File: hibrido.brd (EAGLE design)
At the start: 84 x 80 mm, 30 parts

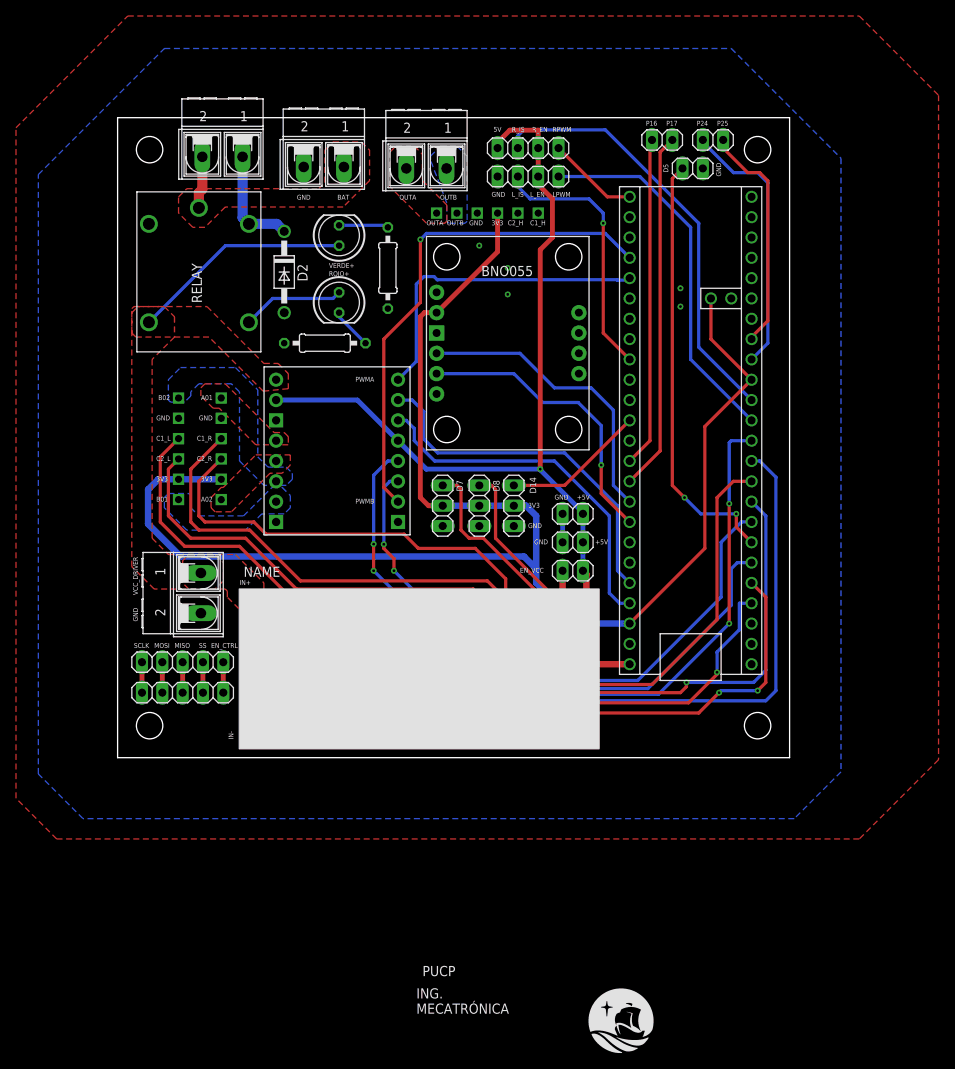
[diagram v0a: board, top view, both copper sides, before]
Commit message: Version final de la PCB, falta revisar por los demás
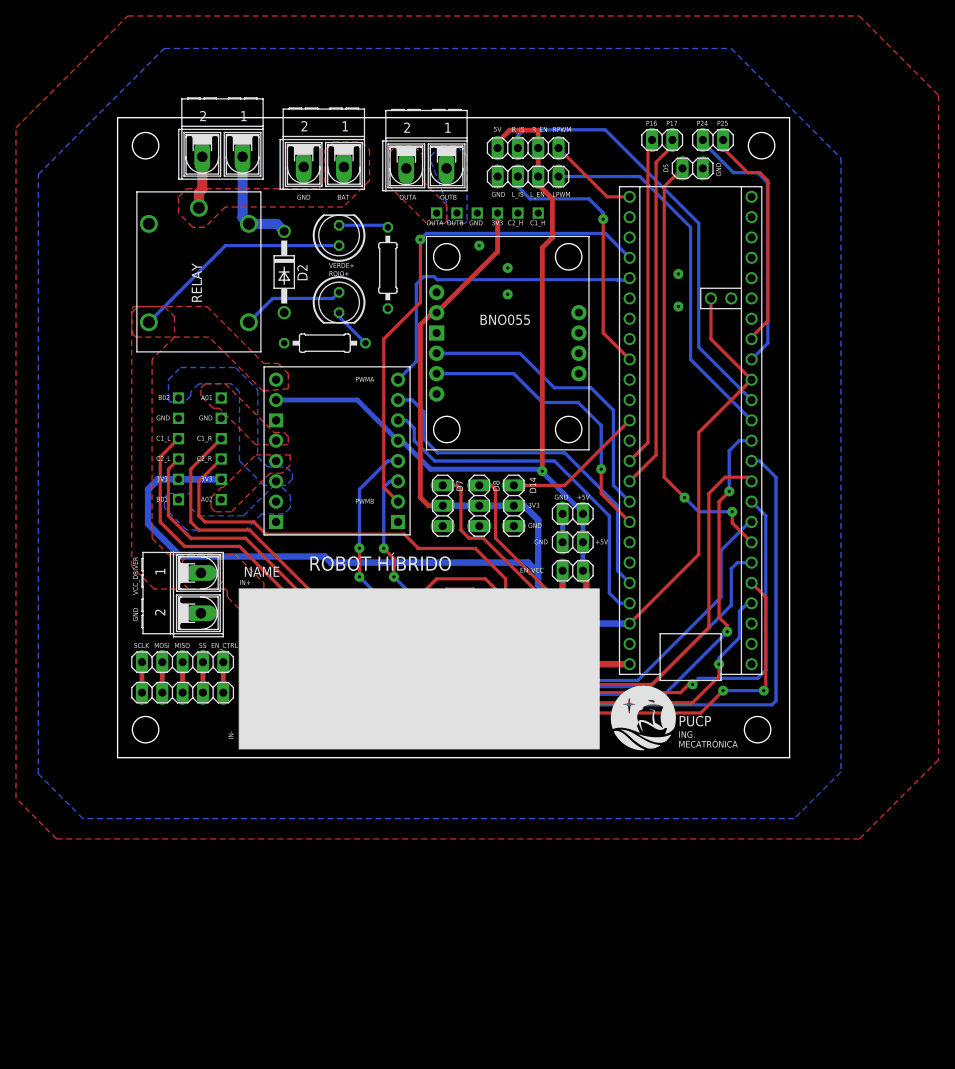
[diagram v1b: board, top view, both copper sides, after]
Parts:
- renumbered U$2 to REG
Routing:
- net BI1: track 103.8 -> 108.0 mm
- net C2_L: track 99.7 -> 102.1 mm
- net C1_R: track 115.7 -> 117.4 mm
- net 8: track 72.3 -> 73.6 mm
- net BI2: track 90.5 -> 91.6 mm
- net C1_L: track 105.7 -> 106.6 mm
- net 5: track 54.0 -> 54.7 mm
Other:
- board text added: "ROBOT HÍBRIDO"

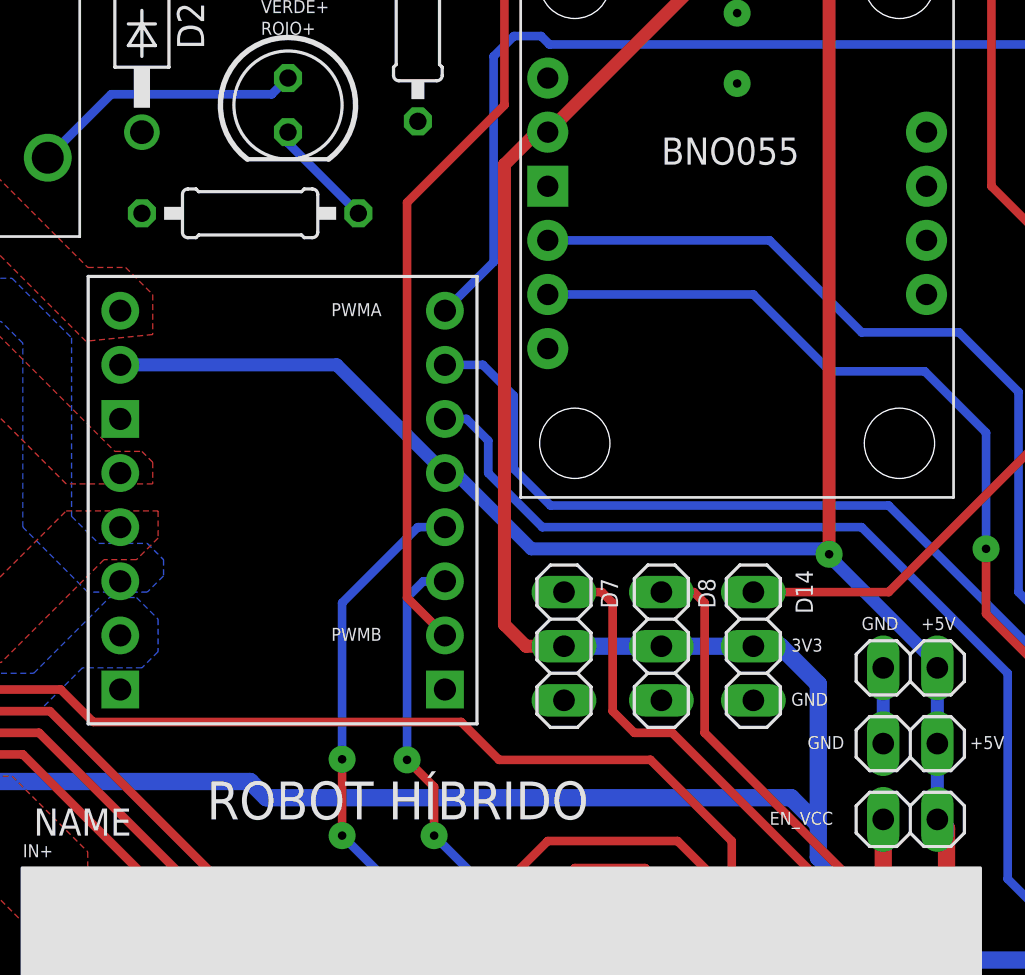
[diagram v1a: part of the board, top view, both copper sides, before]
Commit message: Cambios finales con los nombres
xd
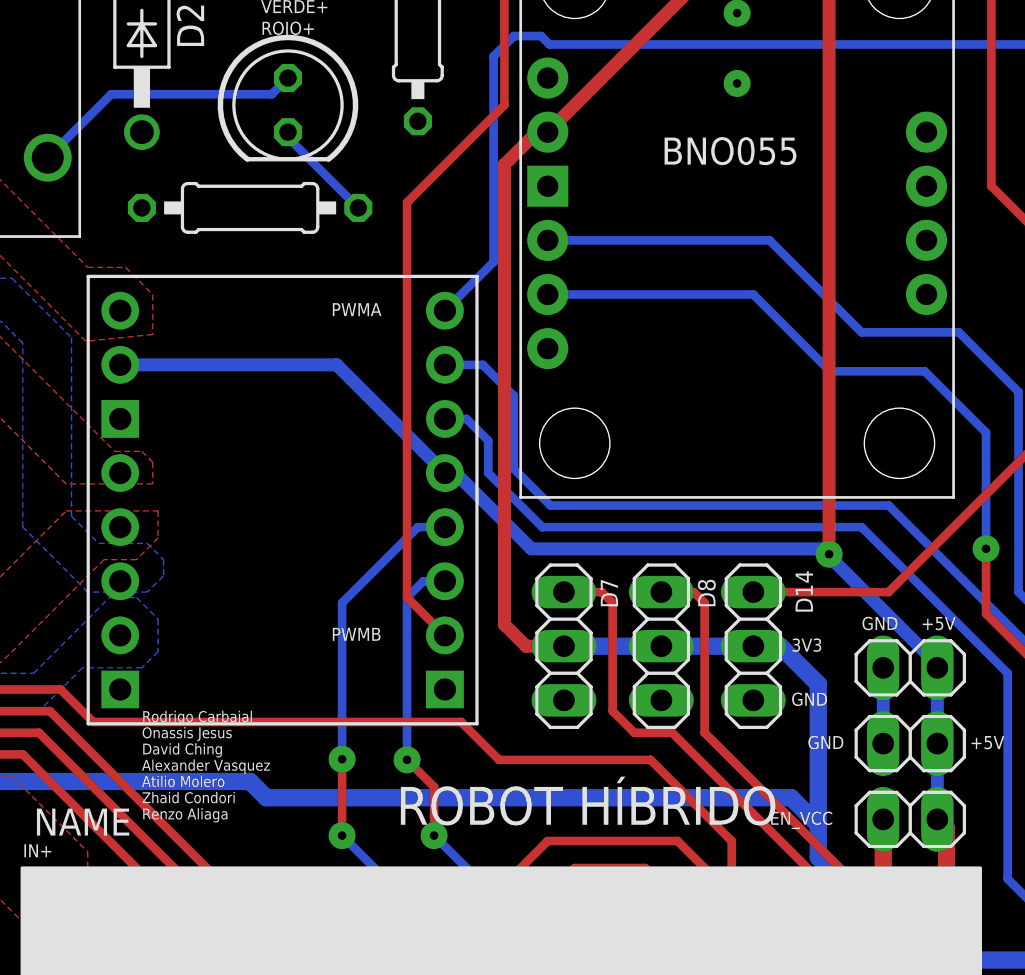
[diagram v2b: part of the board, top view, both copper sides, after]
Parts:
- moved R1 0.25 mm to (25.9, 52.1)
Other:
- board text added: "Rodrigo Carbajal Onassis Jesus David Ching Alexander Vasquez Atilio Molero Zhaid Condori Renzo Aliaga"
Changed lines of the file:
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@@
 <setting verticaltext="up"/>
 </settings>
-<grid distance="10" unitdist="mil" unit="mm" style="lines" multiple="1" display="yes" altdistance="5" altunitdist="mil" altunit="mil"/>
+<grid distance="10" unitdist="mil" unit="mil" style="lines" multiple="1" display="yes" altdistance="5" altunitdist="mil" altunit="mil"/>
 <layers>
 <layer number="1" name="Top" color="4" fill="1" visible="yes" active="yes"/>
@@
 <text x="68.834" y="73.152" size="0.6096" layer="25" rot="R90">D5</text>
 <text x="75.438" y="72.644" size="0.6096" layer="25" rot="R90">GND</text>
-<text x="23.876" y="23.368" size="1.778" layer="25">ROBOT HÍBRIDO</text>
+<text x="32.766" y="23.114" size="1.778" layer="25">ROBOT HÍBRIDO</text>
+<text x="20.828" y="23.368" size="0.508" layer="25">Rodrigo Carbajal
+Onassis Jesus
+David Ching
+Alexander Vasquez
+Atilio Molero
+Zhaid Condori
+Renzo Aliaga</text>
+<text x="65.532" y="47.498" size="1.016" layer="25"></text>
 </plain>
 <attributes>
@@
 <attribute name="VALUE" x="29.4894" y="68.4784" size="1.27" layer="27" ratio="10" rot="R90"/>
 </element>
-<element name="R1" library="rcl" library_urn="urn:adsk.eagle:library:334" package="0207/10" package3d_urn="urn:adsk.eagle:package:23491/2" value="" x="25.908" y="51.816" smashed="yes">
-<attribute name="POPULARITY" value="36" x="25.908" y="51.816" size="1.778" layer="27" display="off"/>
-<attribute name="SPICEPREFIX" value="R" x="25.908" y="51.816" size="1.778" layer="27" display="off"/>
-<attribute name="VALUE" x="23.6474" y="51.181" size="1.27" layer="27" ratio="10"/>
+<element name="R1" library="rcl" library_urn="urn:adsk.eagle:library:334" package="0207/10" package3d_urn="urn:adsk.eagle:package:23491/2" value="" x="25.908" y="52.07" smashed="yes">
+<attribute name="POPULARITY" value="36" x="25.908" y="52.07" size="1.778" layer="27" display="off"/>
+<attribute name="SPICEPREFIX" value="R" x="25.908" y="52.07" size="1.778" layer="27" display="off"/>
+<attribute name="VALUE" x="23.6474" y="51.435" size="1.27" layer="27" ratio="10"/>
 </element>
 <element name="R2" library="rcl" library_urn="urn:adsk.eagle:library:334" package="0207/10" package3d_urn="urn:adsk.eagle:package:23491/2" value="" x="33.782" y="61.214" smashed="yes" rot="R90">
@@
 <contactref element="R1" pad="2"/>
 <contactref element="LED_RED" pad="K"/>
-<wire x1="30.988" y1="51.816" x2="27.686" y2="55.118" width="0.4064" layer="16"/>
-<wire x1="27.686" y1="55.626" x2="27.686" y2="55.118" width="0.4064" layer="16"/>
+<wire x1="30.988" y1="52.07" x2="27.686" y2="55.372" width="0.4064" layer="16"/>
+<wire x1="27.686" y1="55.626" x2="27.686" y2="55.372" width="0.4064" layer="16"/>
 </signal>
 <signal name="N$4">
